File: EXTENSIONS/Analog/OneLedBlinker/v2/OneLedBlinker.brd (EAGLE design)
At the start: 28 x 63 mm, 8 parts, among them X1 USB-A

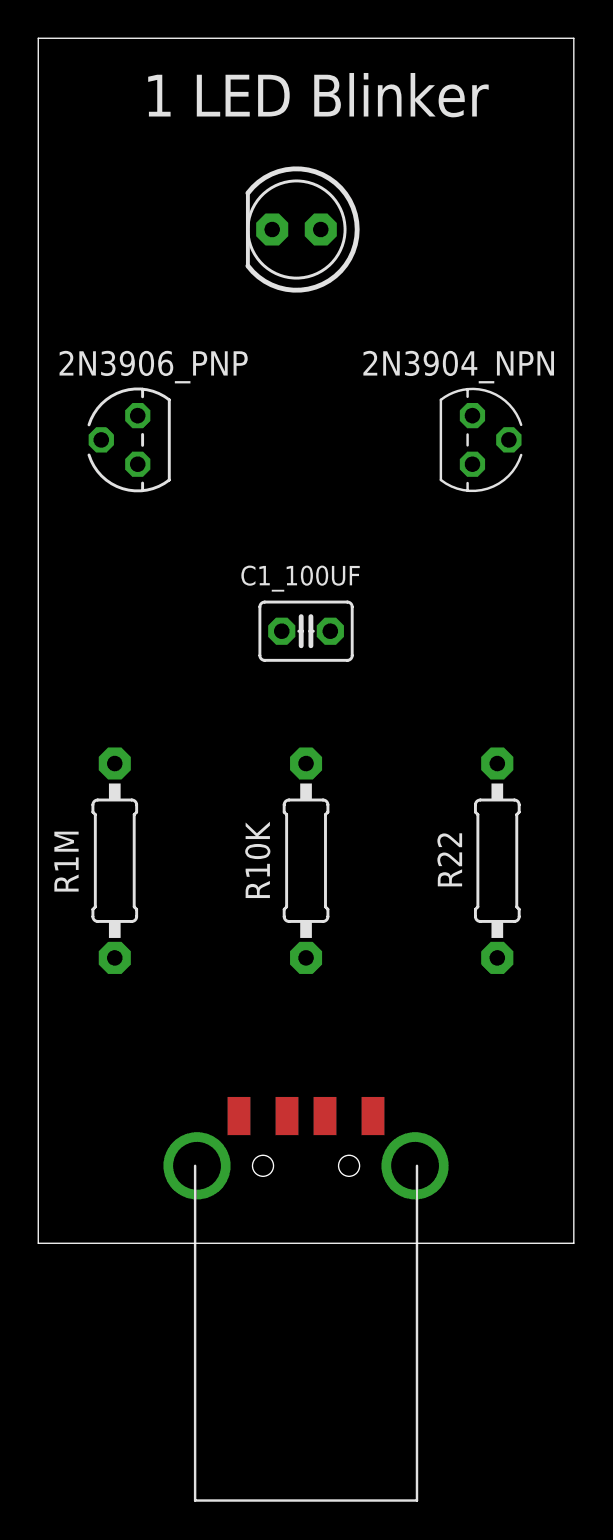
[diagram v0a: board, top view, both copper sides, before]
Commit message: Revisit One Led Blinker pcb
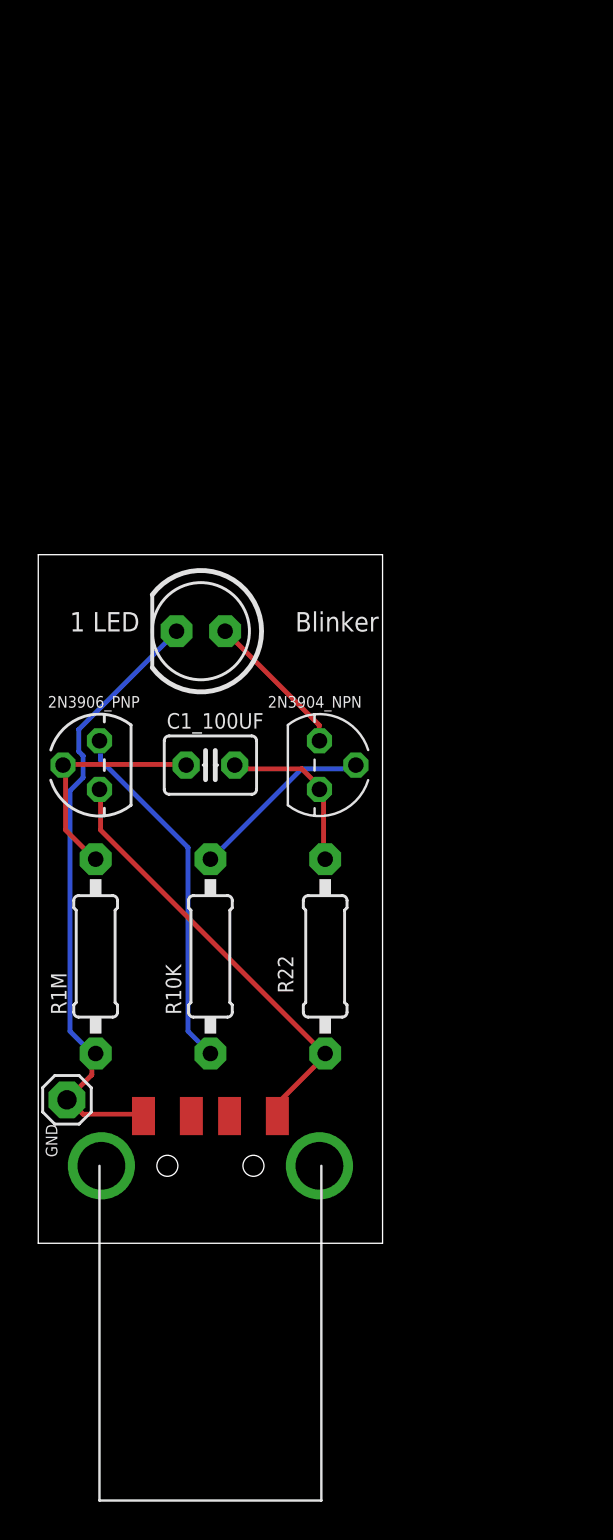
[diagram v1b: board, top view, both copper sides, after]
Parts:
- added GND: GND, adafruit:1X01
- moved LED1 21.6 mm to (10.5, 44.0)
- moved 2N3904_NPN 18.8 mm to (16.7, 37.0)
- moved 2N3906_PNP 17.1 mm to (5.20, 37.0)
- moved R22 10.3 mm to (17.0, 27.0)
- moved C1_100UF 8.60 mm to (11.0, 37.0)
- moved R10K 7.07 mm to (11.0, 27.0)
- moved R1M 5.10 mm to (5.00, 27.0)
- moved X1 5.00 mm to (11.0, 16.1)
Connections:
- net N$4: now also GND.1
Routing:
- net N$4: track 0.00 -> 32.6 mm
- net N$1: track 0.00 -> 23.0 mm
- net N$6: track 0.00 -> 18.7 mm
- net N$5: track 0.00 -> 12.1 mm
- net N$7: track 0.00 -> 9.68 mm
- net N$2: track 0.00 -> 8.92 mm
- net N$3: track 0.00 -> 7.77 mm
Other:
- board size 28 x 63 mm -> 18 x 36 mm
- board text added: "1 LED"
- board text added: "Blinker"
- board text added: "PCBv2 - 2016.10"
- board text added: "www.MadeInTheUSB.net/1LedBlinker"
- board text removed: "1 LED Blinker"
- board text removed: "PCBv3 - 2019.12"
- board text removed: "www.FredericTorres.com"
